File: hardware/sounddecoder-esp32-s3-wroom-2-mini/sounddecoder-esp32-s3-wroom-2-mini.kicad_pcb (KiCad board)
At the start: 4 copper layers, 31.5 x 59.8 mm, 34 parts, among them J1 Input power, J10 AUX1, J101 Conn_01x05, J11 AUX2, J2 Conn_01x02_Pin, J3 Motor, J4 Speaker, J8 FwdLED, J9 BackLED, U1 LM2596S-5, U3 MAX98357A, U4 DRV8251A, U6 AMS1117-3.3, U7 ESP32-S3-WROOM-2, U8 ULN2003A

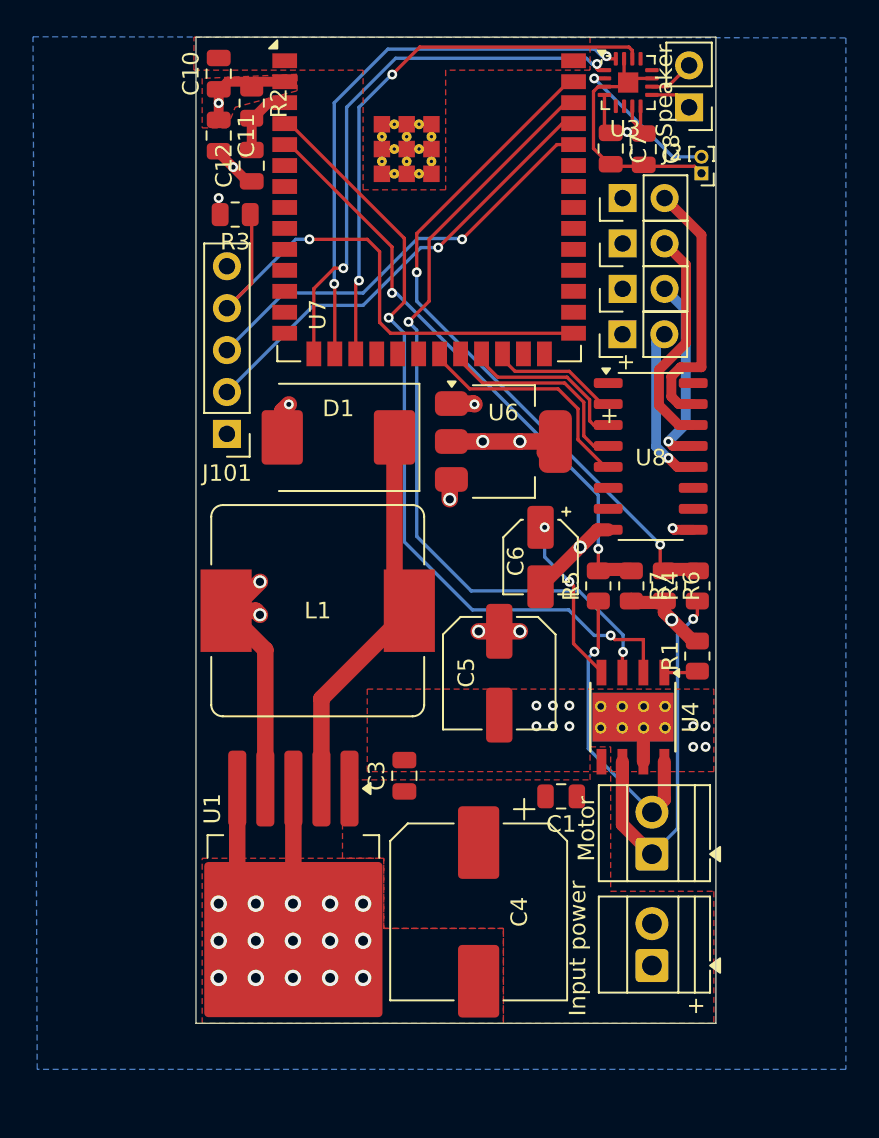
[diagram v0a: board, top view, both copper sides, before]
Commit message: Many updates
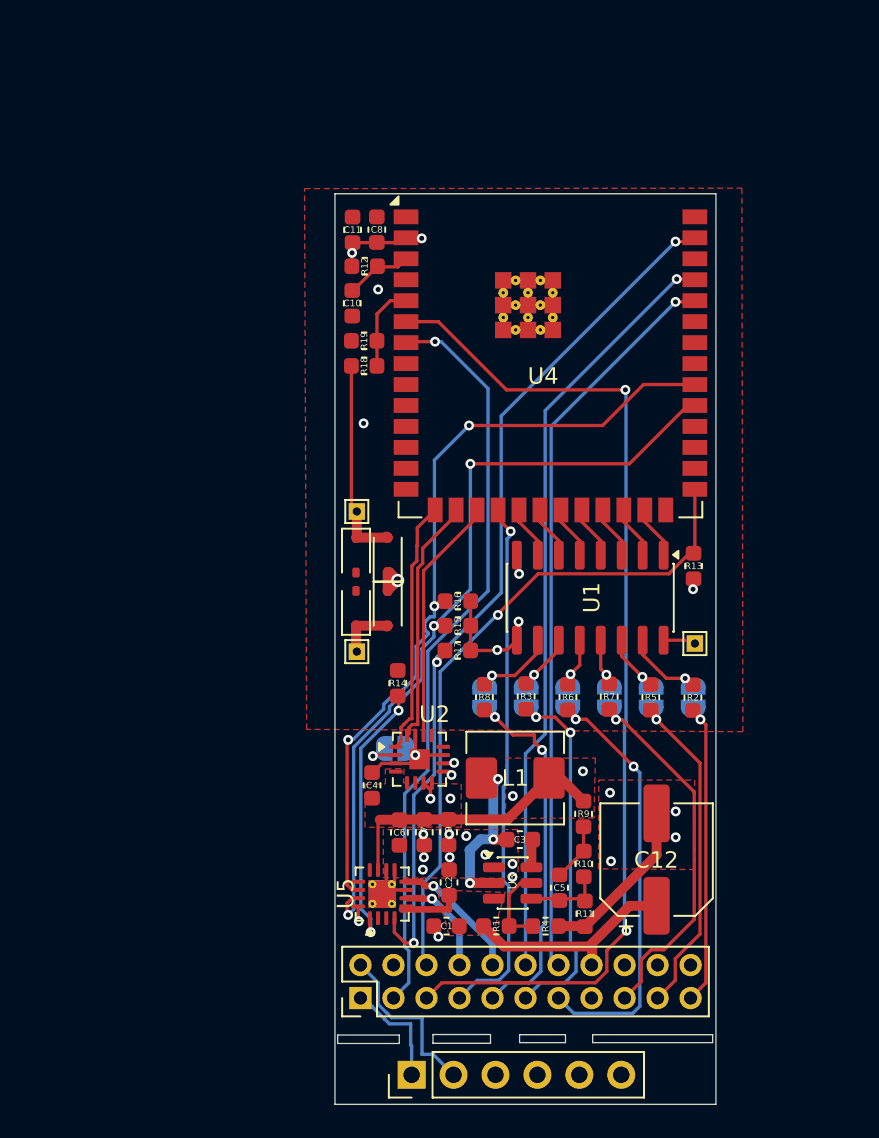
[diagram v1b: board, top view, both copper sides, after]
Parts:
- removed J101: Conn_01x05, Connector_PinHeader_2.54mm:PinHeader_1x05_P2.54mm_Vertical
- removed U6: AMS1117-3.3, Package_TO_SOT_SMD:SOT-223-3_TabPin2
- removed U7: ESP32-S3-WROOM-2, RF_Module:ESP32-S3-WROOM-2
- removed U8: ULN2003A, Package_SO:SO-16_3.9x9.9mm_P1.27mm
- added C2: 0.1uF, Capacitor_SMD:C_0603_1608Metric, F.Cu at (97.2, 127.2)
- added C9: 22uF, Capacitor_SMD:C_0603_1608Metric, F.Cu at (97.2, 124.2)
- added D2: PMEG2020EJ, Diode_SMD:D_SOD-323, F.Cu at (93.5, 107.4)
- added D3: PMEG2020EJ, Diode_SMD:D_SOD-323, F.Cu at (91.6, 107.4)
- added D4: PMEG2020EJ, Diode_SMD:D_SOD-323, F.Cu at (91.6, 110.6)
- added J12: Conn_01x06, Connector_PinHeader_2.54mm:PinHeader_1x06_P2.54mm_Vertical, F.Cu at (94.9, 138.9)
- added J5: Conn_01x02_Pin, Jumper:SolderJumper-2_P1.3mm_Open_RoundedPad1.0x1.5mm, B.Cu at (104.4, 116.0)
- added J6: Conn_01x02_Pin, Jumper:SolderJumper-2_P1.3mm_Open_RoundedPad1.0x1.5mm, B.Cu at (109.5, 116.0)
- added J7: Conn_01x02_Pin, Jumper:SolderJumper-2_P1.3mm_Open_RoundedPad1.0x1.5mm, B.Cu at (93.9, 119.1)
- added R10: 100k, Capacitor_SMD:C_0603_1608Metric, F.Cu at (105.4, 126.1)
- added R11: 22.1k, Capacitor_SMD:C_0603_1608Metric, F.Cu at (105.4, 129.1)
- added R12: 10k, Capacitor_SMD:C_0603_1608Metric, F.Cu at (92.1, 89.9)
- added R13: 10k, Capacitor_SMD:C_0603_1608Metric, F.Cu at (112.0, 108.0)
- added R14: 511, Capacitor_SMD:C_0603_1608Metric, F.Cu at (94.1, 115.1)
- added R15: 2.2k, Capacitor_SMD:C_0603_1608Metric, F.Cu at (97.7, 111.7)
- added R16: 2.2k, Capacitor_SMD:C_0603_1608Metric, F.Cu at (97.7, 110.2)
- added R17: 10k, Capacitor_SMD:C_0603_1608Metric, F.Cu at (97.7, 113.2)
- added R18: 75kΩ, Capacitor_SMD:C_0603_1608Metric, F.Cu at (92.1, 95.9)
- added R19: 12kΩ, Capacitor_SMD:C_0603_1608Metric, F.Cu at (92.1, 94.4)
- added R8: 30, Capacitor_SMD:C_0603_1608Metric, F.Cu at (99.3, 116.0)
- added R9: 49.9, Capacitor_SMD:C_0603_1608Metric, F.Cu at (105.4, 123.1)
- added U2: MAX98357A, Package_DFN_QFN:TQFN-16-1EP_3x3mm_P0.5mm_EP1.23x1.23mm, F.Cu at (95.4, 119.7)
- added U5: DRV8235, Package_DFN_QFN:WQFN-16-1EP_3x3mm_P0.5mm_EP1.68x1.68mm_ThermalVias, F.Cu at (93.2, 127.9)
- C1: value 0.1uF -> 10uF; footprint Capacitor_SMD:C_0805_2012Metric -> Capacitor_SMD:C_0603_1608Metric
- C10: value 0.1uF -> 1uF; footprint Capacitor_SMD:C_0805_2012Metric -> Capacitor_SMD:C_0603_1608Metric
- C11, C3, C8: footprint Capacitor_SMD:C_0805_2012Metric -> Capacitor_SMD:C_0603_1608Metric
- C12: value 1uF -> 47uF; footprint Capacitor_SMD:C_0805_2012Metric -> Capacitor_SMD:CP_Elec_6.3x5.4
- C4: value 470uF -> 0.1uF; footprint Capacitor_SMD:CP_Elec_10x10.5 -> Capacitor_SMD:C_0603_1608Metric
- C5: value 220uF -> 47pF; footprint Capacitor_SMD:C_Elec_6.3x7.7 -> Capacitor_SMD:C_0603_1608Metric
- C6: value 22uF -> 10uF; footprint Capacitor_SMD:CP_Elec_4x5.4 -> Capacitor_SMD:C_0603_1608Metric
- C7: value 10uF -> 22uF; footprint Capacitor_SMD:C_0805_2012Metric -> Capacitor_SMD:C_0603_1608Metric
- D1: value SS54 -> PMEG2020EJ; footprint Diode_SMD:D_SMC -> Diode_SMD:D_SOD-323
- J1: value Input power -> TrackLeft; footprint TerminalBlock:TerminalBlock_Xinya_XY308-2.54-2P_1x02_P2.54mm_Horizontal -> TestPoint:TestPoint_THTPad_1.0x1.0mm_Drill0.5mm
- J10: value AUX1 -> Smoke_Pin; footprint Connector_PinHeader_2.54mm:PinHeader_1x02_P2.54mm_Vertical -> TestPoint:TestPoint_THTPad_1.0x1.0mm_Drill0.5mm
- J11: value AUX2 -> Conn_02x11_Odd_Even; footprint Connector_PinHeader_2.54mm:PinHeader_1x02_P2.54mm_Vertical -> Connector_PinHeader_2.00mm:PinHeader_2x11_P2.00mm_Vertical
- J2: value Conn_01x02_Pin -> TrackRight; footprint Connector_PinHeader_1.00mm:PinHeader_1x02_P1.00mm_Vertical -> TestPoint:TestPoint_THTPad_1.0x1.0mm_Drill0.5mm
- J3: value Motor -> Conn_01x02_Pin; footprint TerminalBlock:TerminalBlock_Xinya_XY308-2.54-2P_1x02_P2.54mm_Horizontal -> Jumper:SolderJumper-2_P1.3mm_Open_RoundedPad1.0x1.5mm; moved to B.Cu
- J4: value Speaker -> Conn_01x02_Pin; footprint Connector_PinHeader_2.54mm:PinHeader_1x02_P2.54mm_Vertical -> Jumper:SolderJumper-2_P1.3mm_Open_RoundedPad1.0x1.5mm; moved to B.Cu
- J8: value FwdLED -> Conn_01x02_Pin; footprint Connector_PinHeader_2.54mm:PinHeader_1x02_P2.54mm_Vertical -> Jumper:SolderJumper-2_P1.3mm_Open_RoundedPad1.0x1.5mm; moved to B.Cu
- J9: value BackLED -> Conn_01x02_Pin; footprint Connector_PinHeader_2.54mm:PinHeader_1x02_P2.54mm_Vertical -> Jumper:SolderJumper-2_P1.3mm_Open_RoundedPad1.0x1.5mm; moved to B.Cu
- L1: value 47uh/L39 -> 6.8uH; footprint Inductor_SMD:L_Bourns_SRP1245A -> Inductor_SMD:L_Chilisin_BMRA00050530
- R1: value 1k -> 511k; footprint Resistor_SMD:R_0805_2012Metric -> Capacitor_SMD:C_0603_1608Metric
- R2, R3: value 10k -> 30; footprint Resistor_SMD:R_0805_2012Metric -> Capacitor_SMD:C_0603_1608Metric
- R4: value 20k -> 105k; footprint Resistor_SMD:R_0805_2012Metric -> Capacitor_SMD:C_0603_1608Metric
- R5: value 20k -> 30; footprint Resistor_SMD:R_0805_2012Metric -> Capacitor_SMD:C_0603_1608Metric
- R6, R7: value 1k -> 30; footprint Resistor_SMD:R_0805_2012Metric -> Capacitor_SMD:C_0603_1608Metric
- U1: value LM2596S-5 -> ULN2003A; footprint Package_TO_SOT_SMD:TO-263-5_TabPin3 -> Package_SO:SO-16_3.9x9.9mm_P1.27mm
- U3: value MAX98357A -> TPS54302; footprint Package_DFN_QFN:TQFN-16-1EP_3x3mm_P0.5mm_EP1.23x1.23mm -> Package_TO_SOT_SMD:SOT-23-6
- U4: value DRV8251A -> ESP32-S3-WROOM-2; footprint Package_SO:Texas_HSOP-8-1EP_3.9x4.9mm_P1.27mm_ThermalVias -> RF_Module:ESP32-S3-WROOM-2
- moved U3 49.0 mm to (101.1, 127.2)
- moved C12 48.7 mm to (109.8, 125.8)
- moved R2 44.9 mm to (112.0, 116.0)
- moved J11 43.2 mm to (91.8, 134.2)
- moved C7 42.9 mm to (95.7, 124.2)
- moved J4 35.7 mm to (112.0, 116.0), turned to 90 degrees
- moved R3 34.1 mm to (101.9, 115.9), turned to -90 degrees
- moved J8 31.4 mm to (99.4, 116.0), turned to -90 degrees
- moved J2 29.3 mm to (91.6, 104.7)
- moved J9 27.5 mm to (106.9, 116.0)
- moved U1 26.3 mm to (105.8, 110.0)
- moved J1 26.1 mm to (91.6, 113.2), turned to 180 degrees
- moved U4 25.5 mm to (103.3, 92.1), turned to 0 degrees
- moved R4 22.6 mm to (103.1, 129.9), turned to 0 degrees
- moved J10 21.9 mm to (112.1, 112.7)
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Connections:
- C10 pad 1: +3.3V -> GND
- C10 pad 2: GND -> Net-(U4-EN)
- C12 pad 1: GND -> VCC
- C12 pad 2: Net-(U7-EN) -> GND
- C3 pad 1: VCC -> Net-(U3-BOOT)
- C3 pad 2: GND -> Net-(U3-SW)
- C4 pad 1: VCC -> +3.3V
- C5 pad 1: +5V -> Net-(C5-Pad1)
- C5 pad 2: GND -> Net-(U3-FB)
- D1 pad 1: /Out5V -> VCC
- D1 pad 2: GND -> /Track_Left
- J1 pad 1: VCC -> /Track_Left
- J10 pad 1: +5V -> /SmokeOn
- J11 pad 1: +5V -> /SOUND1
- J11 pad 2: Net-(J11-Pin_2) -> /SOUND2
- J2 pad 1: GND -> /Track_Right
- J3 pad 1: /MOTOR1 -> Net-(J3-Pin_1)
- J3 pad 2: /MOTOR2 -> /LED5
- J4 pad 1: /Sound1 -> /LED1
- J4 pad 2: /Sound2 -> Net-(J4-Pin_2)
- J8 pad 1: +5V -> Net-(J8-Pin_1)
- J8 pad 2: /FwdLED -> /LED6
- J9 pad 1: +5V -> /LED3
- J9 pad 2: /BackLED -> Net-(J9-Pin_2)
- L1 pad 1: /Out5V -> Net-(U3-SW)
- L1 pad 2: +5V -> +3.3V
- R1 pad 1: Net-(U4-IPROPI) -> VCC
- R1 pad 2: GND -> Net-(U3-EN)
- R2 pad 1: +3.3V -> Net-(J4-Pin_2)
- R2 pad 2: Net-(U7-EN) -> /LED1
- R3 pad 1: /IO0 -> Net-(J3-Pin_1)
- R3 pad 2: +3.3V -> /LED5
- R4 pad 1: /MOTOR1 -> Net-(U3-EN)
- R4 pad 2: /MOTOR_SENSE_1 -> GND
- R5 pad 1: /MOTOR2 -> Net-(J6-Pin_2)
- R5 pad 2: /MOTOR_SENSE_2 -> /LED2
- R6 pad 1: /MOTOR_SENSE_1 -> Net-(J5-Pin_1)
- R6 pad 2: GND -> /LED4
- R7 pad 1: /MOTOR_SENSE_2 -> Net-(J9-Pin_2)
- R7 pad 2: GND -> /LED3
- U1 pad 1: VCC -> /OUT1
- U1 pad 2: /Out5V -> /OUT2
- U1 pad 3: GND -> /OUT3
- U1 pad 4: +5V -> /OUT4
- U1 pad 5: GND -> /OUT5
- U3 pad 1: /AUDIO_OUT -> GND
- U3 pad 2: /SND_GAIN -> Net-(U3-SW)
- U3 pad 3: GND -> VCC
- U3 pad 4: +3.3V -> Net-(U3-FB)
- U3 pad 5: unconnected-(U3-NC-Pad5) -> Net-(U3-EN)
- U3 pad 6: unconnected-(U3-NC-Pad6) -> Net-(U3-BOOT)
- U4 pad 1: Net-(U4-IPROPI) -> GND
- U4 pad 2: /MOTOR_IN2 -> +3.3V
- U4 pad 3: /MOTOR_IN1 -> Net-(U4-EN)
- U4 pad 4: +3.3V -> unconnected-(U4-IO4-Pad4)
- U4 pad 5: VCC -> /DCC
- U4 pad 6: /MOTOR1 -> /GPIO E
- U4 pad 7: GND -> /GPIO D
- U4 pad 8: /MOTOR2 -> /GPIO H
- U4 pad 9: GND -> /GPIO I
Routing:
- net /GPIO E: track 0.00 -> 62.4 mm, vias 0 -> 2
- net VCC: track 0.00 -> 55.1 mm, vias 0 -> 1
- net /MOTOR_FAULT: track 0.00 -> 53.8 mm, vias 0 -> 3
- net /MOTOR_IN1: track 48.2 -> 0.00 mm, vias 2 -> 0
- net /SCL: track 0.00 -> 47.8 mm, vias 0 -> 3
- net /SDA: track 0.00 -> 47.8 mm, vias 0 -> 3
- net /MOTOR_IN2: track 47.6 -> 0.00 mm, vias 2 -> 0
- net /UART-TX/GPIO A: track 0.00 -> 46.5 mm, vias 0 -> 1
- net /GPIO D: track 0.00 -> 45.7 mm, vias 0 -> 1
- net /UART-RX/GPIO B: track 0.00 -> 44.7 mm, vias 0 -> 1
- net /MOTOR_SENSE_1: track 41.9 -> 0.00 mm, vias 2 -> 0
- net /BOOT/GPIO C: track 0.00 -> 40.4 mm, vias 0 -> 1
- net /MOTOR_SENSE_2: track 35.9 -> 0.00 mm, vias 2 -> 0
- net /IO0: track 33.9 -> 0.00 mm, vias 1 -> 0
- net /GPIO F: track 0.00 -> 32.2 mm, vias 0 -> 1
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- removed copper zone on In2.Cu, net +5V
- removed copper zone on B.Cu, net GND
- removed copper zone on In2.Cu, net VCC
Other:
- board size 31.5 x 59.8 mm -> 23.1 x 55.2 mm
- board text added: "D | +3.3V"
- board text added: "E | BOOT/C"
- board text added: "F | MOTOR1"
- board text added: "GND | VCC"
- board text added: "LED1"
- board text added: "LED1 | +3.3V"
- board text added: "LED2"
- board text added: "LED2 | +3.3V"
- board text added: "LED3"
- board text added: "LED3 | +3.3V"
- board text added: "LED4"
- board text added: "LED4 | RX/B"
- board text added: "LED5"
- board text added: "LED5 | TX/A"
- board text added: "LED6"
- board text added: "LED6 | MOTOR2"
- board text added: "MRRSoundDecoder mini v3.0 2026 Dovgalyuk P."
- board text added: "SOUND1 | SOUND2"
- board text added: "SmokeOn"
- board text added: "SndGain"
- board text added: "Track"
- board text removed: "+"
- board text removed: "+5V"
- board text removed: "-"
- board text removed: "AUX1"
- board text removed: "AUX2"
- board text removed: "BOOT"
- board text removed: "BackLED"
- board text removed: "FwdLED"
- board text removed: "GND"
- board text removed: "RX"
- board text removed: "TX"
